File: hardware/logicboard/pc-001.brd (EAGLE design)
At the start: 25 x 61.5 mm, 17 parts, among them J4 DNP, J5 DNP

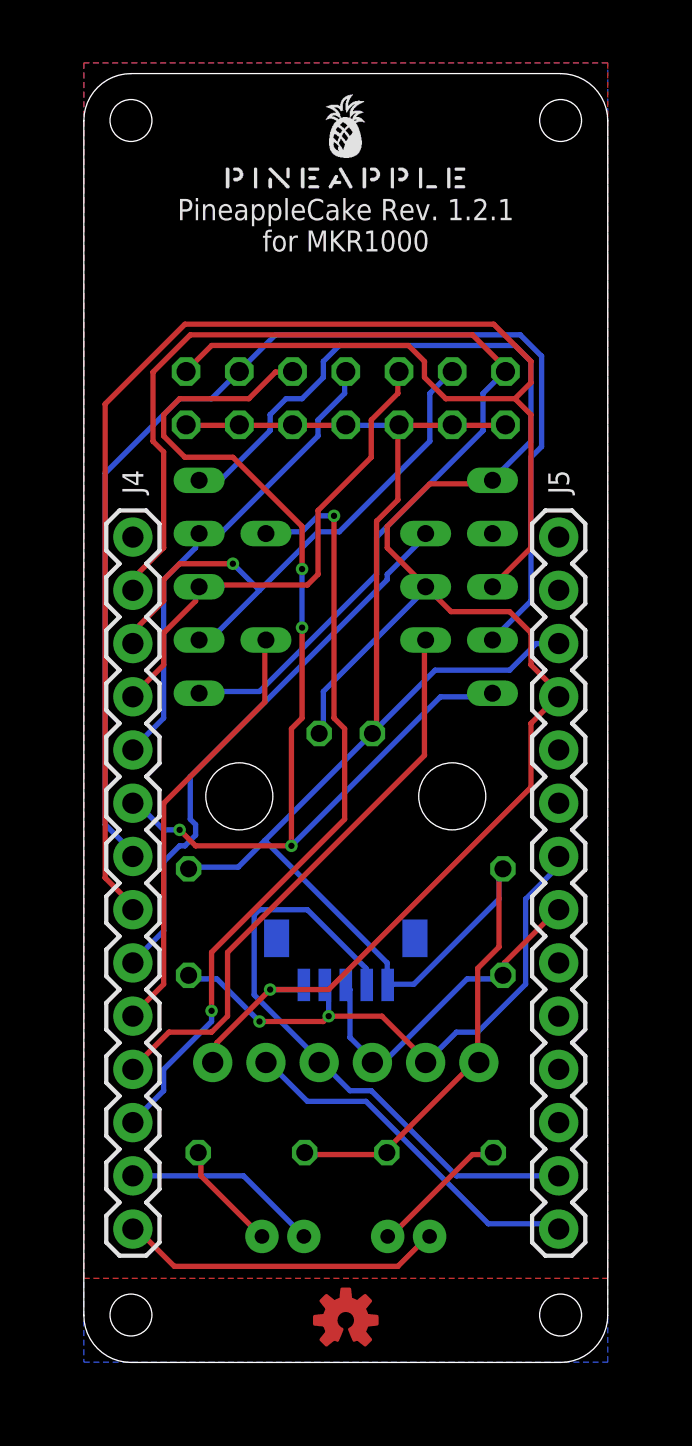
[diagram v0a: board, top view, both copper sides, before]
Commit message: Rerouted.
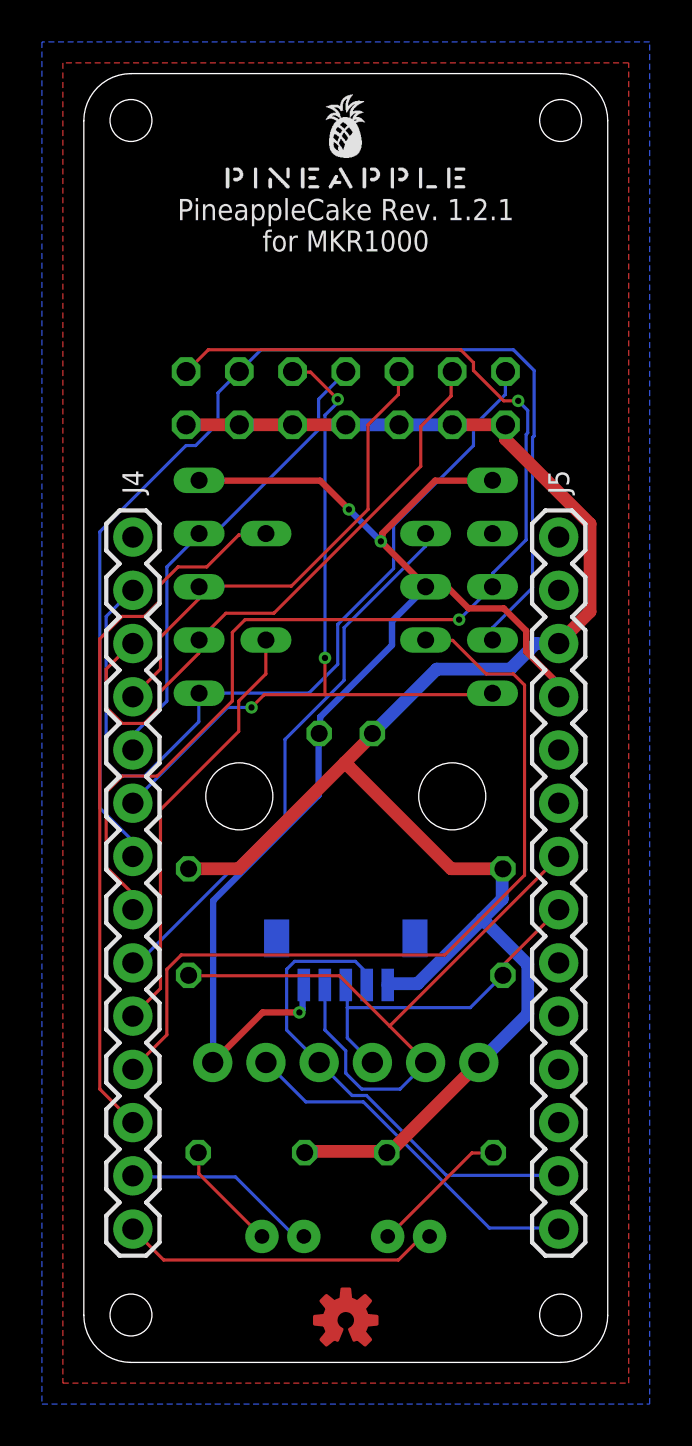
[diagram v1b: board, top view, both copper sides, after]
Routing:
- net GND: track 82.0 -> 62.5 mm, vias 1 -> 3
- net A6: track 77.1 -> 57.8 mm, vias 0 -> 2
- net A4: track 52.9 -> 36.4 mm, vias 4 -> 3
- net A0: track 52.6 -> 40.3 mm
- net D2: track 27.4 -> 39.0 mm
- net D7: track 29.4 -> 23.5 mm
- net SDA: track 28.0 -> 33.8 mm, vias 2 -> 0
- net VCC: track 90.7 -> 87.2 mm
- net D3: track 36.9 -> 34.2 mm, vias 2 -> 0
- net A1: track 27.8 -> 30.0 mm, vias 1 -> 0
- net A5: track 57.3 -> 55.4 mm
